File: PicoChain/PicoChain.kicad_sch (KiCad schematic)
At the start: 14 parts, among them J1 RJ45, J2 RJ45, J3 Conn_01x02_Socket, J4 Conn_01x02_Socket, J5 Conn_01x20_Socket, J6 Conn_01x20_Socket, U1 PCA9615DP, U2 RASPBERRY_PI_PICO

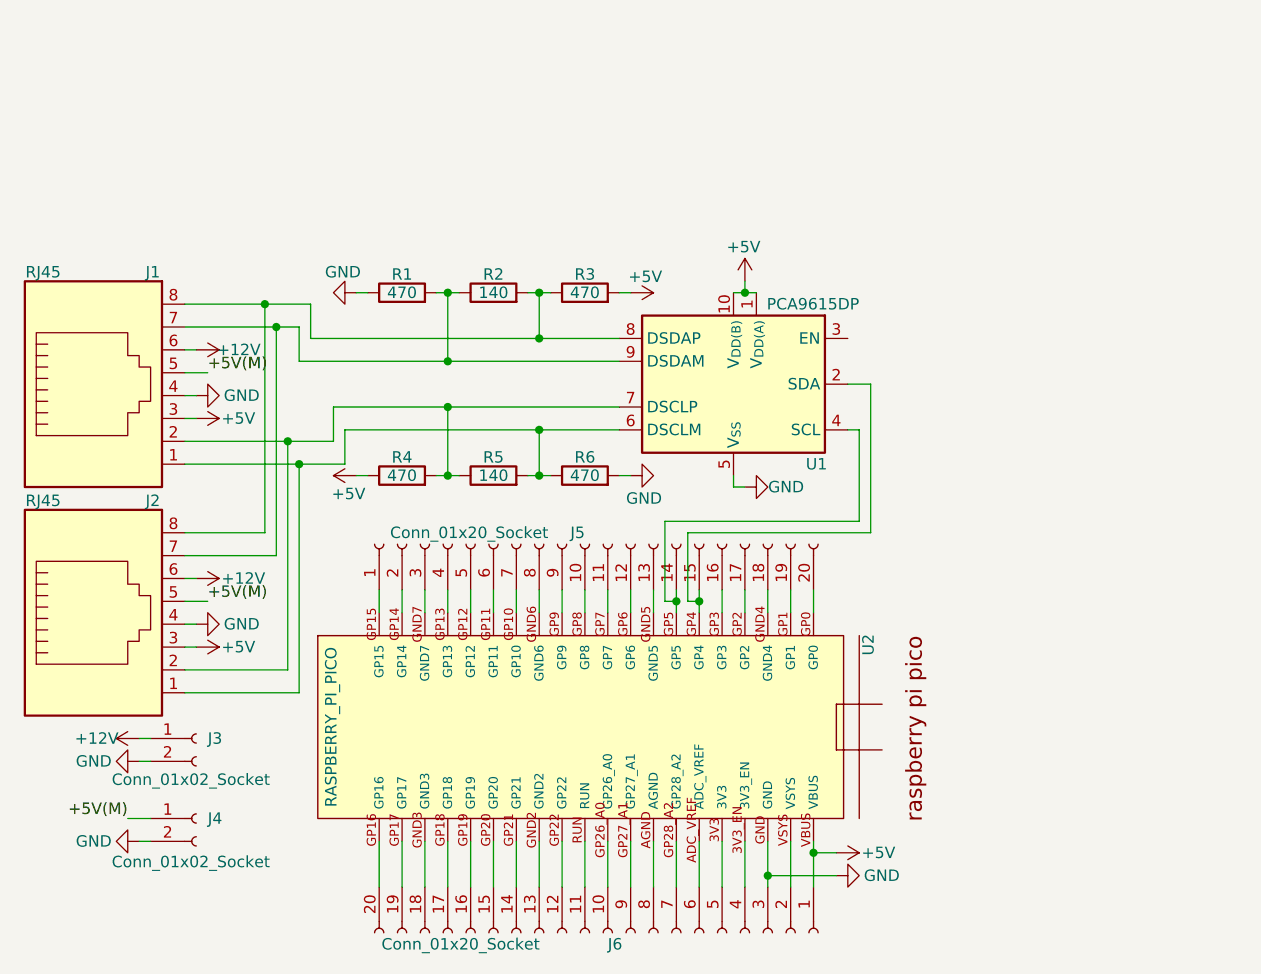
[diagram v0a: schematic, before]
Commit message: Updated to version 1.1
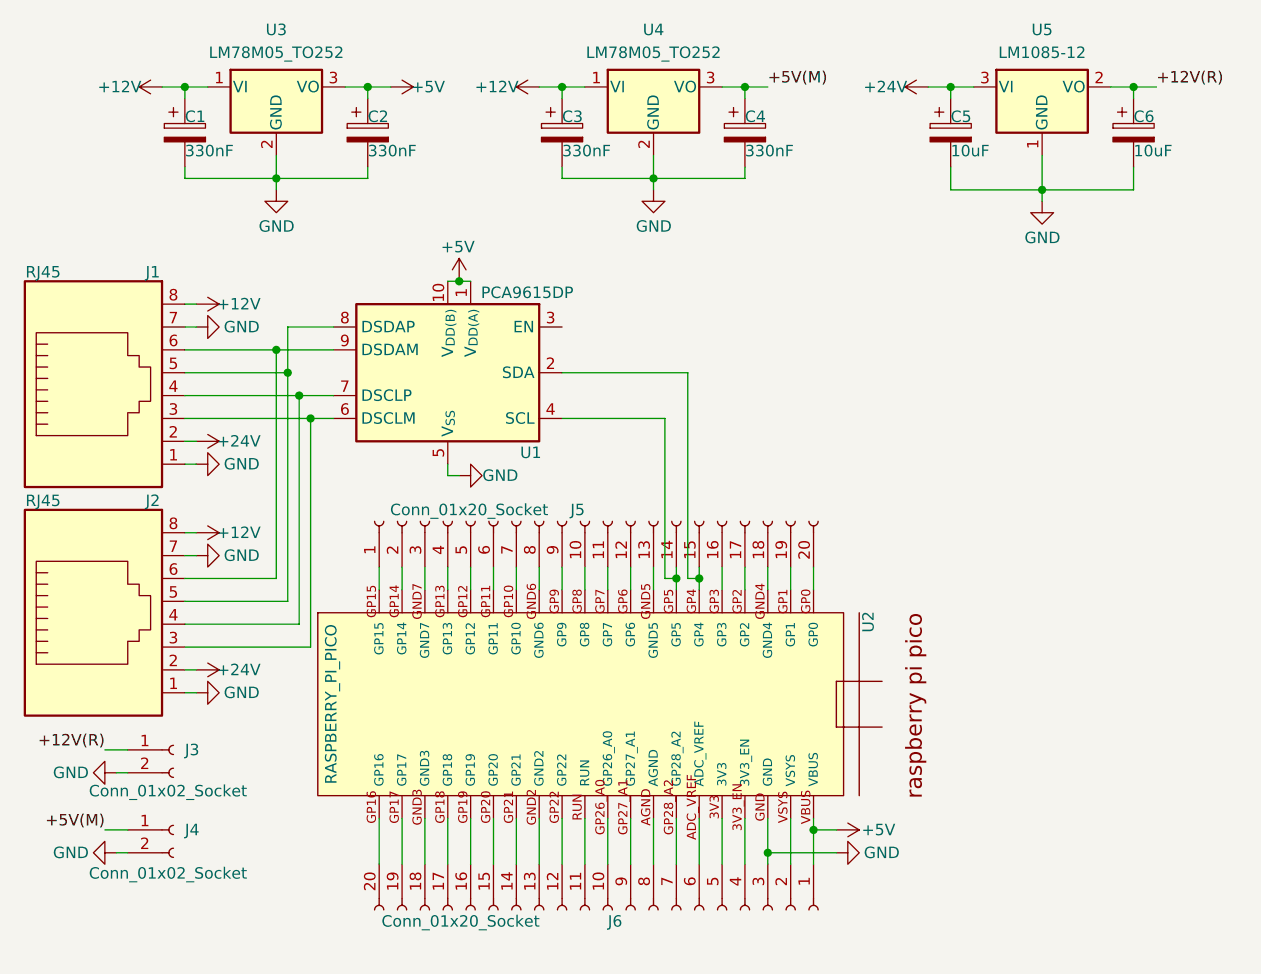
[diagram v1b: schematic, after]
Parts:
- removed R1, R3, R4, R6: 470, Resistor_SMD:R_0805_2012Metric, symbol Device:R
- removed R2, R5: 140, Resistor_SMD:R_0805_2012Metric, symbol Device:R
- added C1, C2, C3, C4: 330nF, Capacitor_Tantalum_SMD:CP_EIA-3216-18_Kemet-A, symbol Device:C_Polarized
- added C5, C6: 10uF, Capacitor_Tantalum_SMD:CP_EIA-3528-21_Kemet-B, symbol Device:C_Polarized
- added U3, U4: LM78M05_TO252, Package_TO_SOT_SMD:TO-252-2, symbol Regulator_Linear:LM78M05_TO252
- added U5: LM1085-12, LM1085IS-12:TO254P1524X483-4N, symbol Regulator_Linear:LM1085-12
- U2: footprint MCU_RaspberryPi_and_Boards:RPi_Pico_SMD_TH -> RASPBERRY_PI_PICO:RASPBERRY_PI_PICO
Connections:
- net +12V: now also J1.8, J2.8, C1.1, C3.1, U3.1 (VI), U4.1 (VI); no longer J1.6, J2.6, J3.1 (Pin_1)
- net +5V: now also C2.1, U3.3 (VO); no longer J1.3, J2.3
- net +5V(M): now also C4.1, U4.3 (VO); no longer J1.5, J2.5
- net GND: now also J1.1, J1.7, J2.1, J2.7, C1.2, C2.2, C3.2, C4.2, C5.2, C6.2, U3.2 (GND), U4.2 (GND), U5.1 (GND); no longer J1.4, J2.4
- net +24V: now reaches J1.2, J2.2
- net +24V: now also C5.1, U5.3 (VI); no longer U1.7 (DSCLP)
- new net: J1.3, J2.3, U1.6 (DSCLM)
- new net: J1.4, J2.4, U1.7 (DSCLP)
- new net: J1.5, J2.5, U1.8 (DSDAP)
- new net: J1.6, J2.6, U1.9 (DSDAM)
- new net +12V(R): C6.1, J3.1 (Pin_1), U5.2 (VO)
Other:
- moved on the sheet: J3, J4, J5, J6, U1, U2
